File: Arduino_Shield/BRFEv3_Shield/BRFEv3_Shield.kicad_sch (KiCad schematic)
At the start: 8 parts, among them P1 Power, P2 Analog, P3 Digital, P4 Digital, P5 CONN_01X01, P6 CONN_01X01, P7 CONN_01X01, P8 CONN_01X01

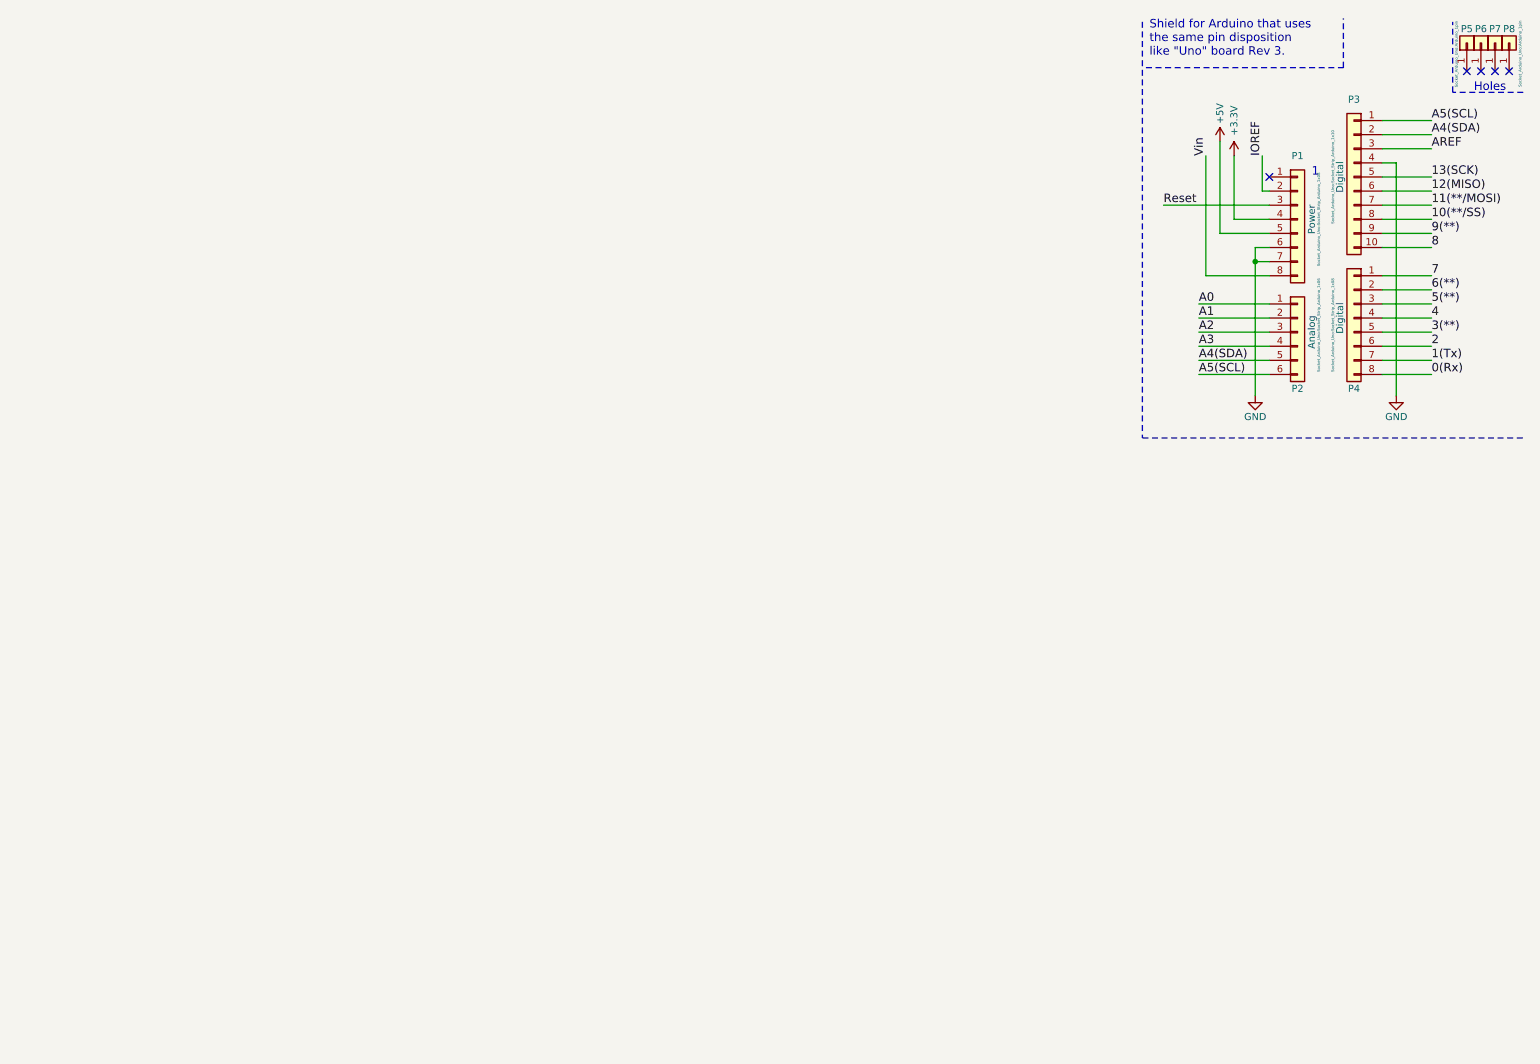
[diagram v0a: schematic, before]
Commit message: update shield
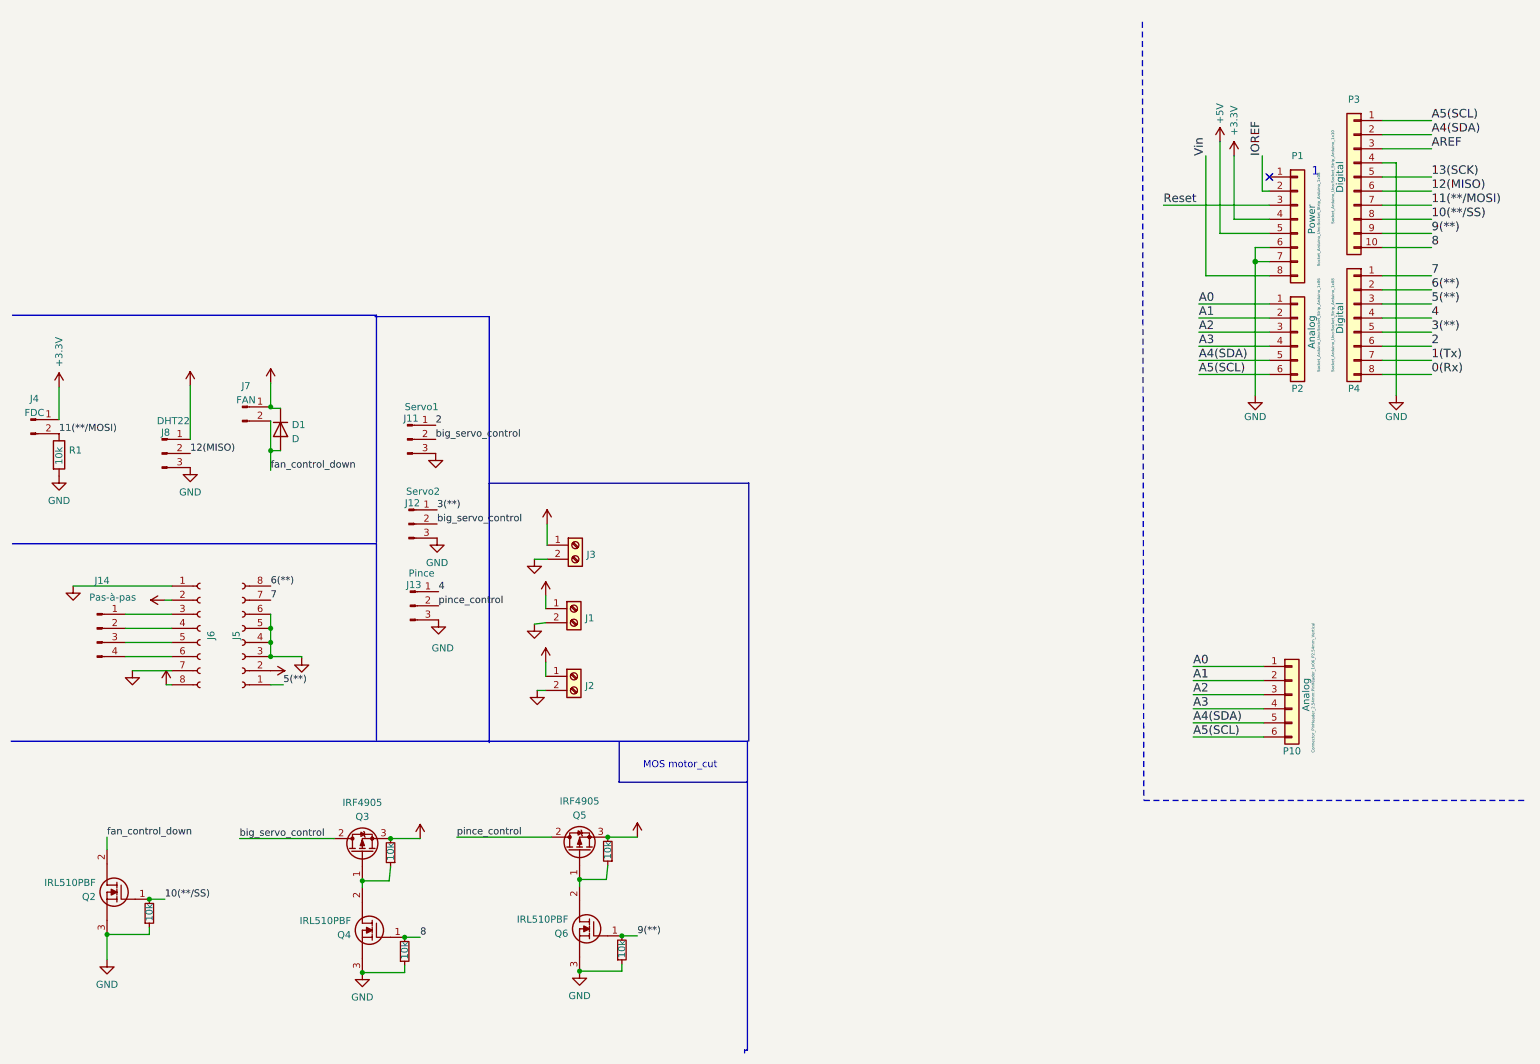
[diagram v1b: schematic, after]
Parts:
- removed P5, P6, P7, P8: CONN_01X01, Socket_Arduino_Uno:Arduino_1pin, symbol Connector_Generic:Conn_01x01
- added D1: D, Diode_THT:D_DO-41_SOD81_P3.81mm_Vertical_AnodeUp, symbol Device:D
- added J1, J2, J3: Screw_Terminal_01x02, Connector_Phoenix_MSTB:PhoenixContact_MSTBVA_2,5_2-G_1x02_P5.00mm_Vertical, symbol Connector:Screw_Terminal_01x02
- added J11: Servo1, Connector_PinHeader_2.54mm:PinHeader_1x03_P2.54mm_Vertical, symbol Connector:Conn_01x03_Male
- added J12: Servo2, Connector_PinHeader_2.54mm:PinHeader_1x03_P2.54mm_Vertical, symbol Connector:Conn_01x03_Male
- added J13: Pince, Connector_PinHeader_2.54mm:PinHeader_1x03_P2.54mm_Vertical, symbol Connector:Conn_01x03_Male
- added J14: Pas-à-pas, Connector_PinHeader_2.54mm:PinHeader_1x04_P2.54mm_Vertical, symbol Connector:Conn_01x04_Male
- added J4: FDC, Connector_PinHeader_2.54mm:PinHeader_1x02_P2.54mm_Vertical, symbol Connector:Conn_01x02_Male
- added J5, J6: Conn_01x08_Female, Connector_PinHeader_2.54mm:PinHeader_1x08_P2.54mm_Vertical, symbol Connector:Conn_01x08_Female
- added J7: FAN, Connector_PinHeader_2.54mm:PinHeader_1x02_P2.54mm_Vertical, symbol Connector:Conn_01x02_Male
- added J8: DHT22, Connector_PinHeader_2.54mm:PinHeader_1x03_P2.54mm_Vertical, symbol Connector:Conn_01x03_Male
- added P10: Analog, Connector_PinHeader_2.54mm:PinHeader_1x06_P2.54mm_Vertical, symbol Connector_Generic:Conn_01x06
- added Q2, Q4, Q6: IRL510PBF, Package_TO_SOT_THT:TO-220-3_Vertical, symbol IRL510PBF:IRL510PBF
- added Q3, Q5: IRF4905, Package_TO_SOT_THT:TO-220-3_Vertical, symbol Transistor_FET:IRF4905
- added R1: 10k, Resistor_THT:R_Axial_DIN0204_L3.6mm_D1.6mm_P5.08mm_Vertical, symbol Device:R
- added R3, R4, R5, R6, R7: 10k, Resistor_THT:R_Axial_DIN0204_L3.6mm_D1.6mm_P5.08mm_Vertical, symbol Device:R_Small
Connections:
- net +3V3: now also J4.1 (Pin_1)
- net +5V: now also J2.1 (Pin_1), J5.2 (Pin_2), J6.2 (Pin_2), J8.1 (Pin_1), Q5.3 (S), R6.2
- net 12(MISO): now also J8.2 (Pin_2)
- net 2: now also J11.1 (Pin_1)
- net 3(**): now also J12.1 (Pin_1)
- net 4: now also J13.1 (Pin_1)
- net 5(**): now also J5.1 (Pin_1)
- net 6(**): now also J5.8 (Pin_8)
- net 7: now also J5.7 (Pin_7)
- net 8: now also Q4.1, R5.2
- net 9(**): now also Q6.1, R7.2
- net A0: now also P10.1 (Pin_1)
- net A1: now also P10.2 (Pin_2)
- net A2: now also P10.3 (Pin_3)
- net A3: now also P10.4 (Pin_4)
- net A4(SDA): now also P10.5 (Pin_5)
- net A5(SCL): now also P10.6 (Pin_6)
- net GND: now also J1.2 (Pin_2), J11.3 (Pin_3), J12.3 (Pin_3), J13.3 (Pin_3), J2.2 (Pin_2), J3.2 (Pin_2), J5.3 (Pin_3), J5.4 (Pin_4), J5.5 (Pin_5), J5.6 (Pin_6), J6.1 (Pin_1), J6.7 (Pin_7), J8.3 (Pin_3), Q2.3, Q4.3, Q6.3, R1.2, R3.1, R5.1, R7.1
- new net: Q5.1 (G), Q6.2, R6.1
- new net: J14.1 (Pin_1), J6.3 (Pin_3)
- new net: J14.2 (Pin_2), J6.4 (Pin_4)
- new net: J14.3 (Pin_3), J6.5 (Pin_5)
- new net: J14.4 (Pin_4), J6.6 (Pin_6)
- new net: Q3.1 (G), Q4.2, R4.1
- new net +12V: D1.1 (K), J3.1 (Pin_1), J6.8 (Pin_8), J7.1 (Pin_1)
- new net +6V: J1.1 (Pin_1), Q3.3 (S), R4.2
- new net 10(**/SS): Q2.1, R3.2
- new net 11(**/MOSI): J4.2 (Pin_2), R1.1
- new net big_servo_control: J11.2 (Pin_2), J12.2 (Pin_2), Q3.2 (D)
- new net fan_control_down: D1.2 (A), J7.2 (Pin_2), Q2.2
- new net pince_control: J13.2 (Pin_2), Q5.2 (D)
- no-connect marks 5 -> 1
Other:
- note added: "MOS motor_cut"
- note removed: "Holes"
- note removed: "Shield for Arduino that uses the same pin disposition like "Uno" board Rev 3."
- company: (none) -> Exploradôme
- title: (none) -> Shield Arduino Uno bras robotisé FabriqExpo
